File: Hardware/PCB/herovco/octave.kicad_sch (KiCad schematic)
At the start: 12 parts, among them SW1 SW_Rotary12, SW2 SW_DP3T

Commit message: Big panel and PCB revisions
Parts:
- SW2: footprint (none) -> ao_tht:Heatsink_17x17mm_A-5093
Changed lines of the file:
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@@
     (property "Reference" "SW2" (id 0) (at 209.55 92.2233 0))
     (property "Value" "SW_DP3T" (id 1) (at 209.55 94.9984 0))
-    (property "Footprint" "" (id 2) (at 193.675 94.615 0)
+    (property "Footprint" "ao_tht:Heatsink_17x17mm_A-5093" (id 2) (at 193.675 94.615 0)
       (effects (font (size 1.27 1.27)) hide)
     )
@@
     (property "Reference" "SW2" (id 0) (at 222.25 106.1933 0))
     (property "Value" "SW_DP3T" (id 1) (at 222.25 108.9684 0))
-    (property "Footprint" "" (id 2) (at 206.375 108.585 0)
+    (property "Footprint" "ao_tht:Heatsink_17x17mm_A-5093" (id 2) (at 206.375 108.585 0)
       (effects (font (size 1.27 1.27)) hide)
     )

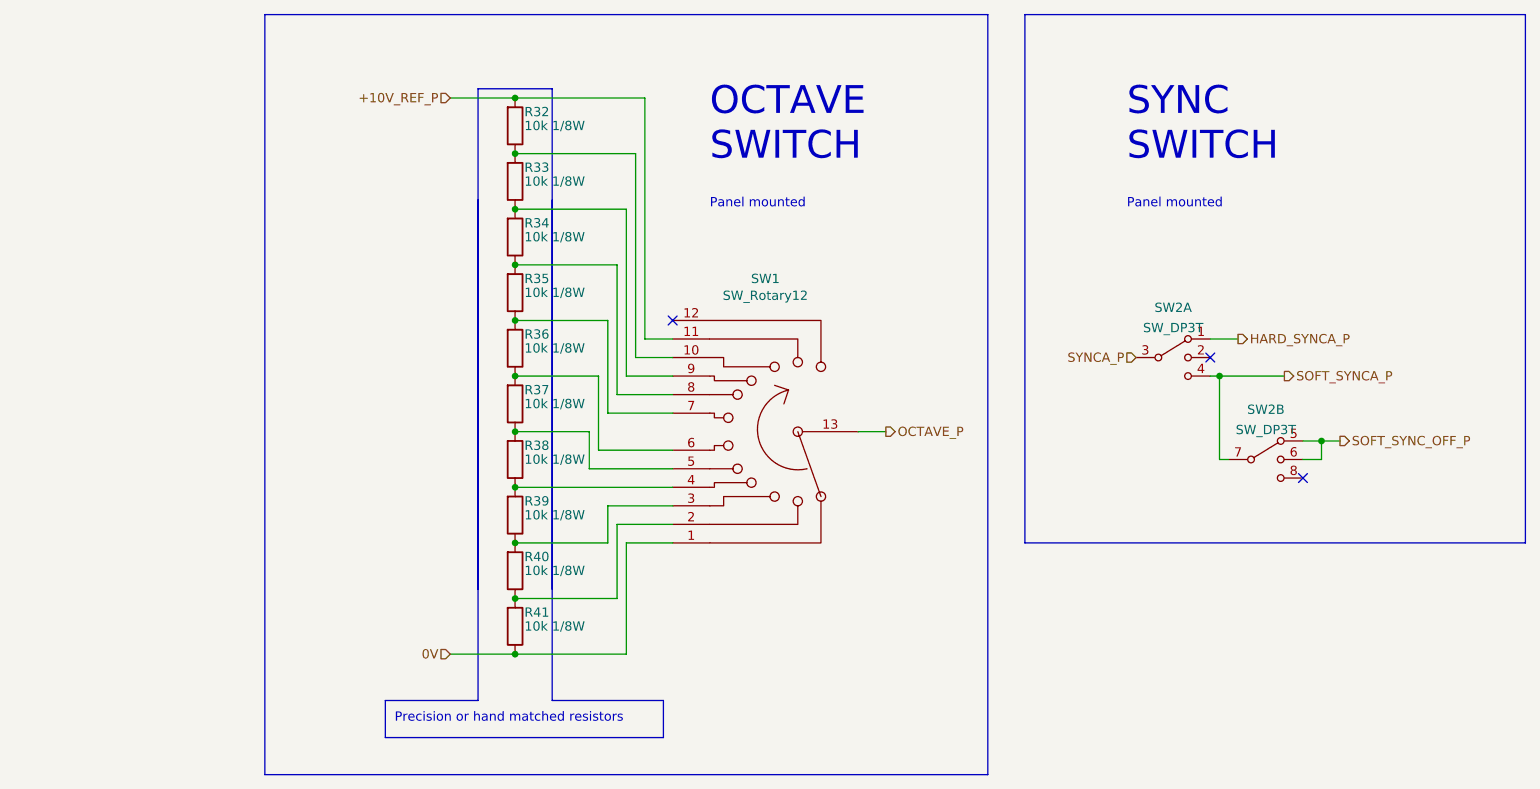
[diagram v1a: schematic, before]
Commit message: Sch cleanup, switch footprint
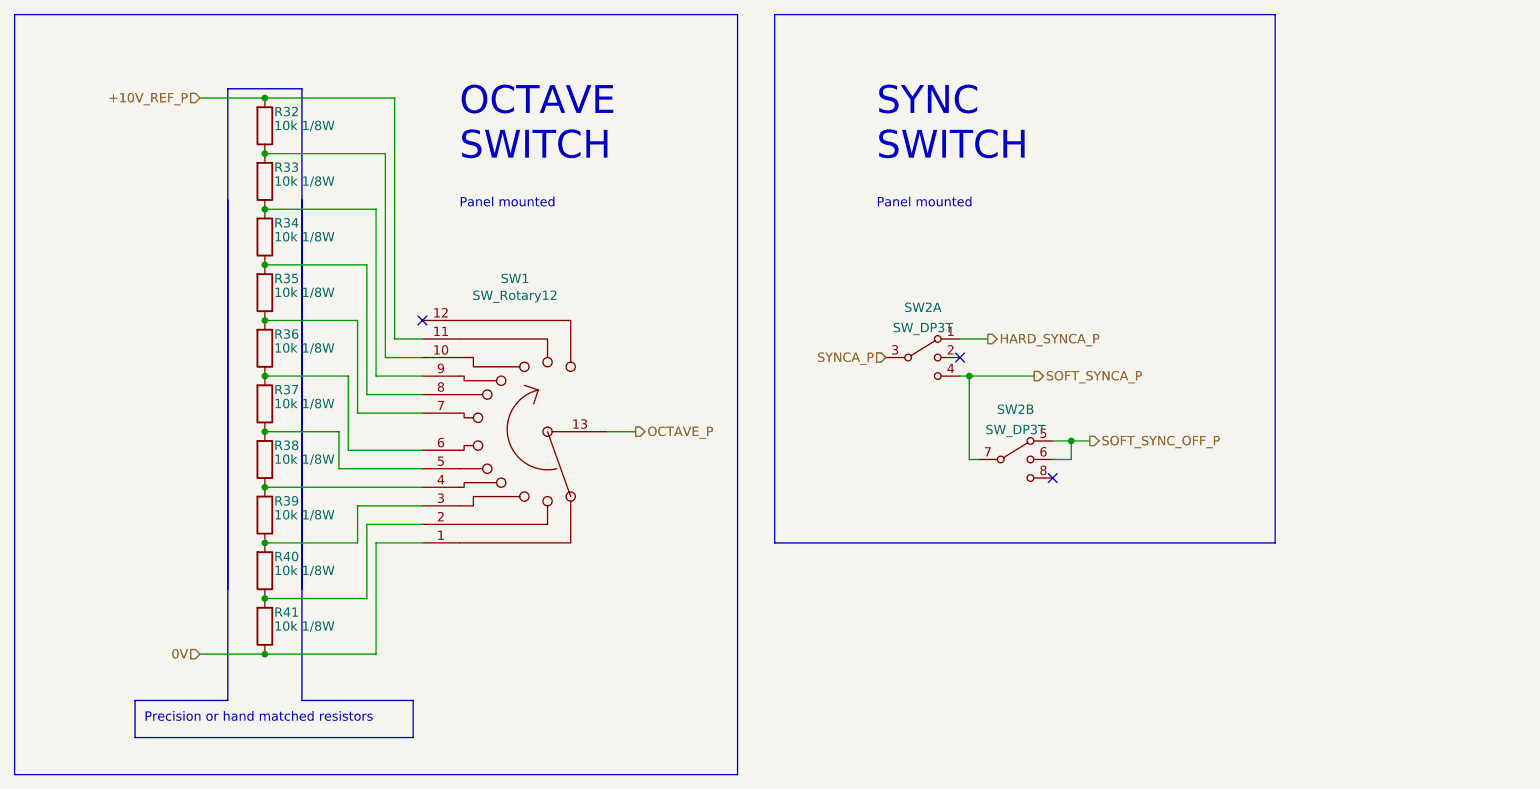
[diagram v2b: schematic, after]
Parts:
- removed SW2: SW_DP3T, ao_tht:Heatsink_17x17mm_A-5093, symbol Switch:SW_DP3T
- added SW2: SW_DP3T, herovco:G-1128S_DP3T, symbol herovco:SW_DP3T
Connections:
- net HARD_SYNCA_P: now also SW2.1
- net SOFT_SYNCA_P: now also SW2.4, SW2.7
- net SOFT_SYNC_OFF_P: now also SW2.5, SW2.6
- net SYNCA_P: now also SW2.3
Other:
- moved on the sheet: R32, R33, R34, R35, R36, R37, R38, R39, R40, R41, SW1
